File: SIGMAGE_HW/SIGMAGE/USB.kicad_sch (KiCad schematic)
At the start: 46 parts, among them J1 UJ31CHG2SMTTR, J3 TSW10607GS, J6 TSW10607GS, U13 ESDR0502NMUTBG, U14 93LC56-I/SN, U9 FT2232HLTRAY

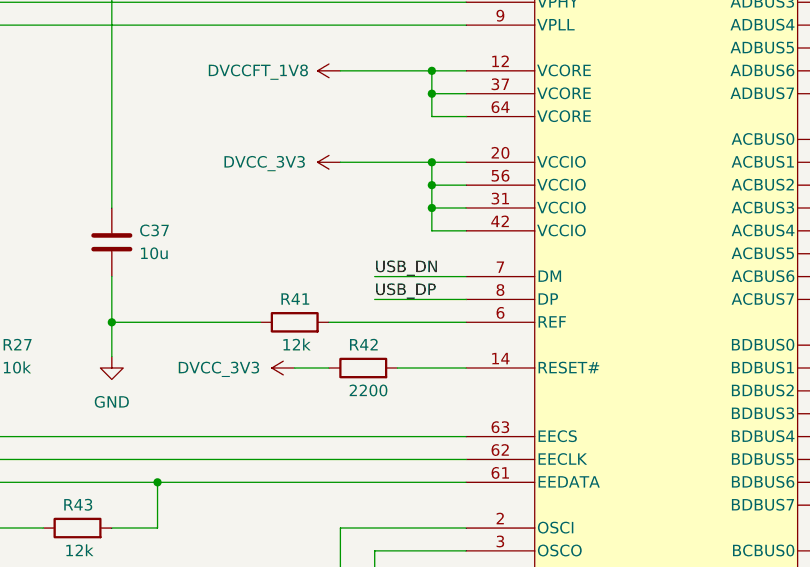
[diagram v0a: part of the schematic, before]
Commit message: stuff
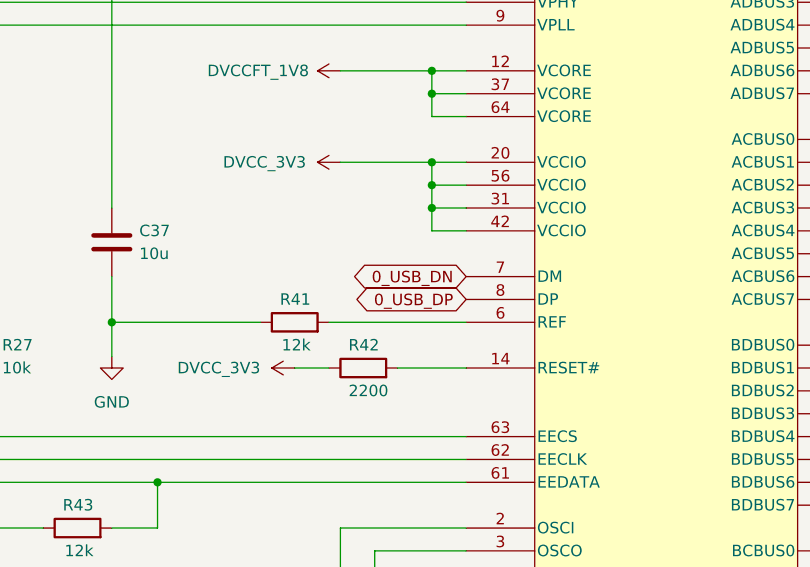
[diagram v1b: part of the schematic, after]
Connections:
- net USB_DN is gone; now on net 0_USB_DN: U9.7 (DM)
- net USB_DP is gone; now on net 0_USB_DP: U9.8 (DP)
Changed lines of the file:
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@@
-	(wire
-		(pts
-			(xy 139.7 165.1) (xy 149.86 165.1)
-		)
-		(stroke
-			(width 0)
-			(type default)
-		)
-	)
 	(wire
 		(pts
@@
 	(wire
 		(pts
-			(xy 139.7 167.64) (xy 149.86 167.64)
-		)
-		(stroke
-			(width 0)
-			(type default)
-		)
-	)
-	(wire
-		(pts
 			(xy 113.03 50.8) (xy 113.03 52.07)
 		)
@@
 			(width 0)
 			(type default)
-		)
-	)
-	(label "USB_DP"
-		(at 139.7 167.64 0)
-		(effects
-			(font
-				(size 1.27 1.27)
-			)
-			(justify left bottom)
 		)
 	)
@@
 				(italic yes)
 				(color 0 0 194 1)
-			)
-			(justify left bottom)
-		)
-	)
-	(label "USB_DN"
-		(at 139.7 165.1 0)
-		(effects
-			(font
-				(size 1.27 1.27)
 			)
 			(justify left bottom)
@@
 		)
 	)
+	(global_label "0_USB_DN"
+		(shape bidirectional)
+		(at 149.86 165.1 180)
+		(fields_autoplaced yes)
+		(effects
+			(font
+				(size 1.27 1.27)
+			)
+			(justify right)
+		)
+		(property "Intersheetrefs" "${INTERSHEET_REFS}"
+			(at 136.2083 165.1 0)
+			(hide yes)
+			(show_name no)
+			(do_not_autoplace no)
+			(effects
+				(font
+					(size 1.27 1.27)
+				)
+				(justify right)
+			)
+		)
+	)
 	(global_label "0_MCU_JTAG_TDI"
 		(shape bidirectional)
@@
 			)
 		)
+	)
+	(global_label "0_USB_DP"
+		(shape bidirectional)
+		(at 149.86 167.64 180)
+		(fields_autoplaced yes)
+		(effects
+			(font
+				(size 1.27 1.27)
+			)
+			(justify right)
+		)
+		(property "Intersheetrefs" "${INTERSHEET_REFS}"
+			(at 136.2688 167.64 0)
+			(hide yes)
+			(show_name no)
+			(do_not_autoplace no)
+			(effects
+				(font
+					(size 1.27 1.27)
+				)
+				(justify right)
+			)
+		)
